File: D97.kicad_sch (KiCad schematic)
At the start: 0 parts

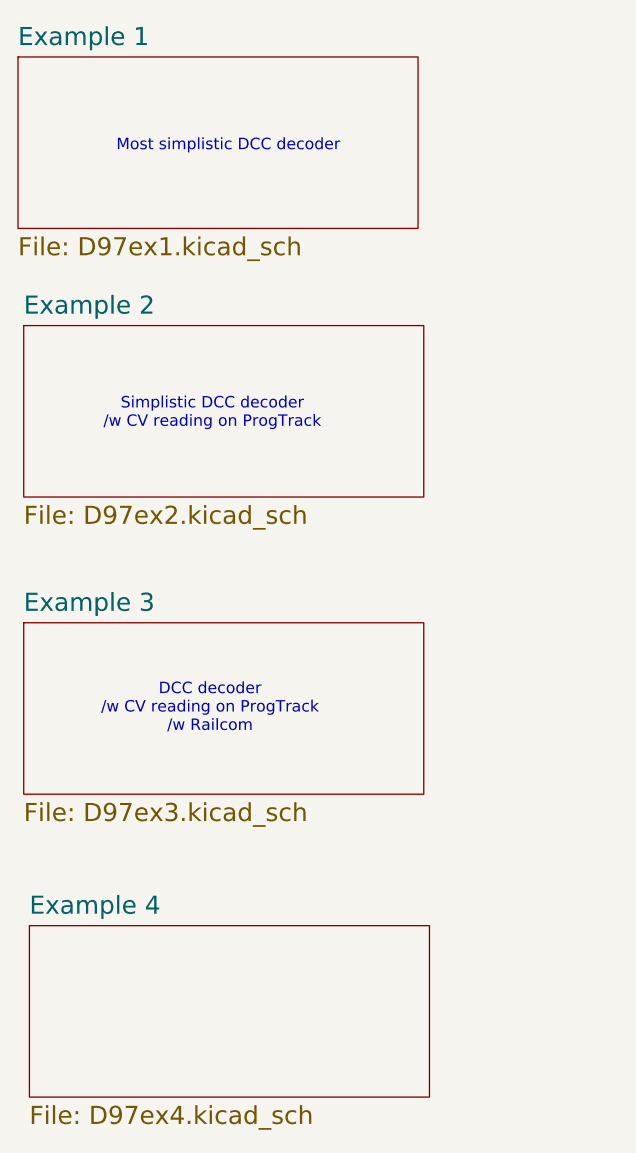
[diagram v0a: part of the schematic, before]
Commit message: initial commit
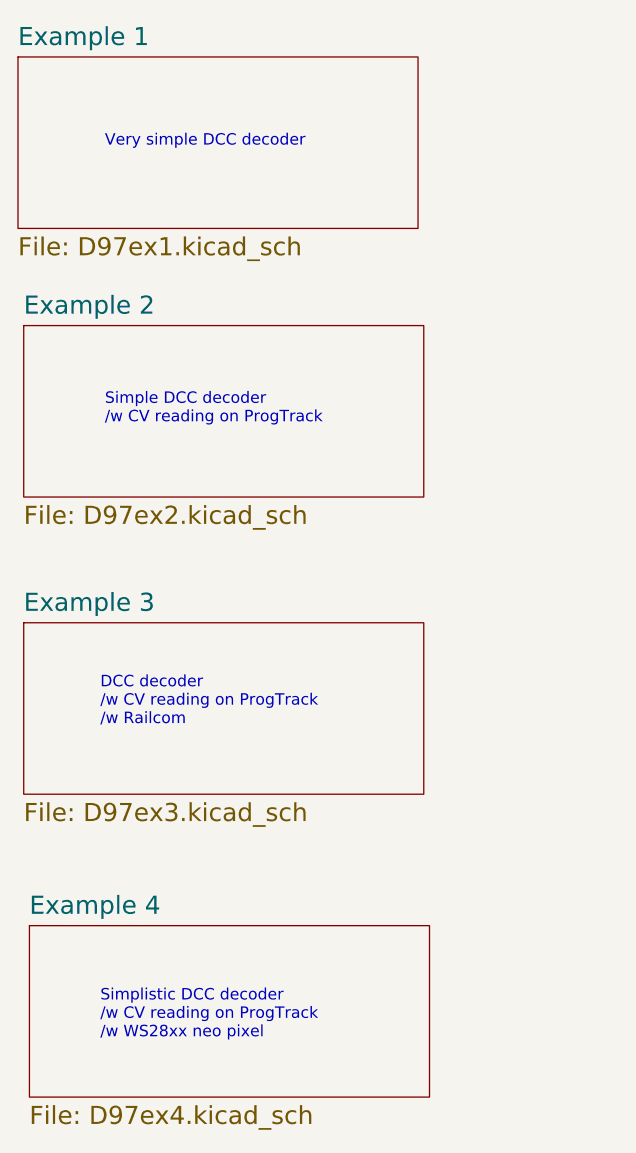
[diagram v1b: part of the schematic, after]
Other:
- note added: "Simple DCC decoder /w CV reading on ProgTrack"
- note added: "Simplistic DCC decoder /w CV reading on ProgTrack /w WS28xx neo pixel"
- note added: "Very simple DCC decoder"
- note removed: "Most simplistic DCC decoder"
- note removed: "Simplistic DCC decoder /w CV reading on ProgTrack"
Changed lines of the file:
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@@
 	(text "DCC decoder\n/w CV reading on ProgTrack\n/w Railcom"
 		(exclude_from_sim no)
-		(at 42.926 95.25 0)
+		(at 30.734 94.488 0)
 		(effects
 			(font
 				(size 1.27 1.27)
 			)
+			(justify left)
 		)
 	)
-	(text "Simplistic DCC decoder\n/w CV reading on ProgTrack"
+	(text "Simple DCC decoder\n/w CV reading on ProgTrack"
 		(exclude_from_sim no)
-		(at 43.18 62.484 0)
+		(at 31.242 61.976 0)
 		(effects
 			(font
 				(size 1.27 1.27)
 			)
+			(justify left)
 		)
 	)
-	(text "Most simplistic DCC decoder"
+	(text "Very simple DCC decoder"
 		(exclude_from_sim no)
-		(at 44.958 32.766 0)
+		(at 31.242 32.258 0)
 		(effects
 			(font
 				(size 1.27 1.27)
 			)
+			(justify left)
 		)
 	)
+	(text "Simplistic DCC decoder\n/w CV reading on ProgTrack\n/w WS28xx neo pixel"
+		(exclude_from_sim no)
+		(at 30.734 129.286 0)
+		(effects
+			(font
+				(size 1.27 1.27)
+			)
+			(justify left)
+		)
+	)
